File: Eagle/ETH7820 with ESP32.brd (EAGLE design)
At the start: 75 x 29.5 mm, 40 parts

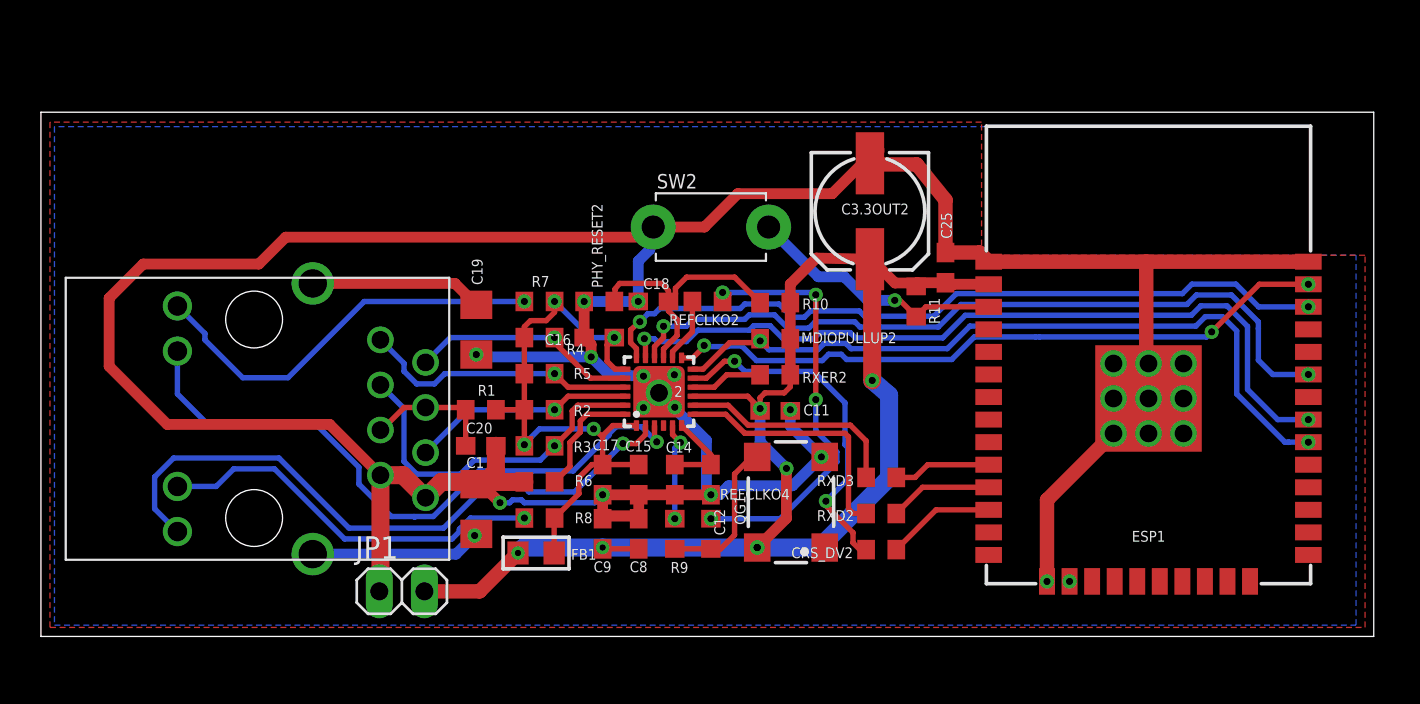
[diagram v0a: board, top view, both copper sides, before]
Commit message: board renew
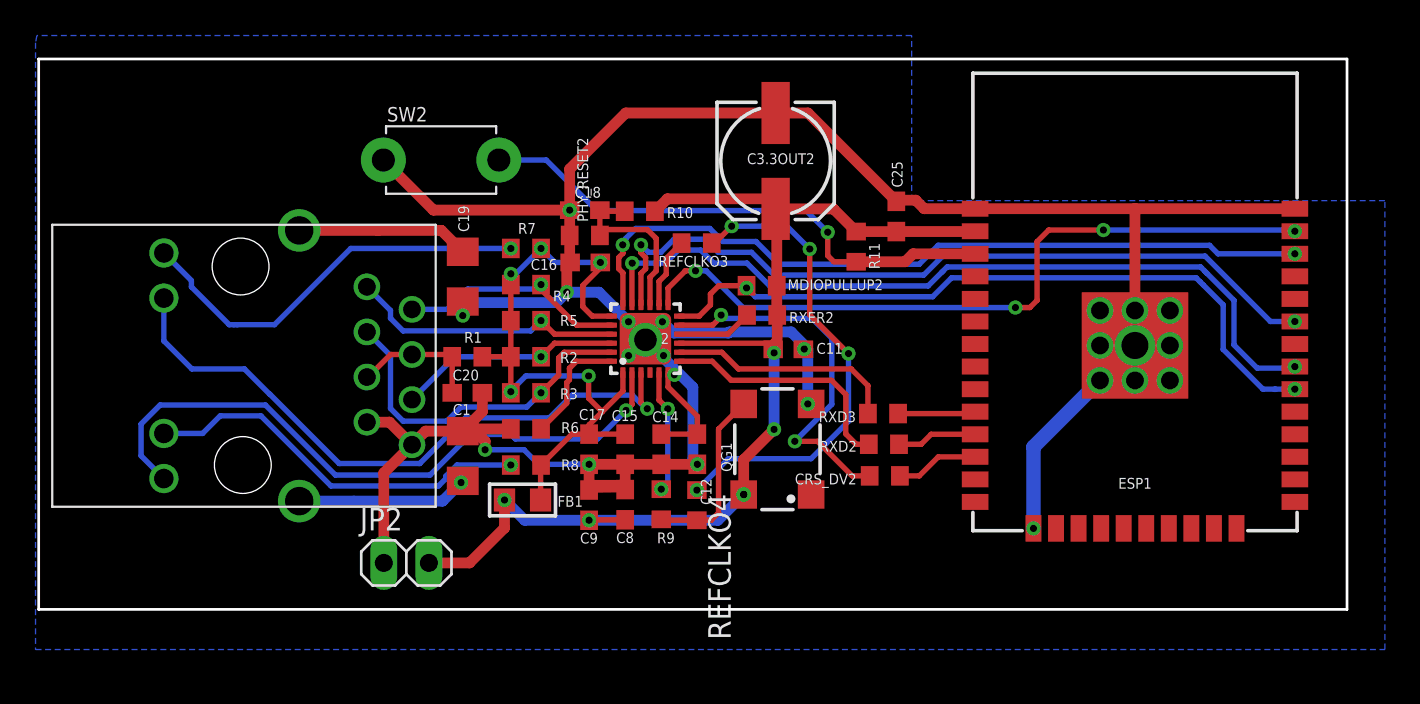
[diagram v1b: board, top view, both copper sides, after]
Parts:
- removed JP1: (no value), pinhead:1X02
- removed REFCLKO2: 33R/1%/R0603, rcl:R0603
- added JP2: (no value), pinhead:1X02
- added REFCLKO3: 33R/1%/R0603, rcl:R0603
- PHY_RESET2: value no value -> do not populate
- moved SW2 15.7 mm to (22.5, 26.8)
- moved R10 9.19 mm to (33.7, 23.9)
- moved C18 6.43 mm to (30.6, 24.0)
- moved C3.3OUT2 6.02 mm to (41.4, 26.8)
- moved R11 4.58 mm to (45.9, 21.9)
- moved C16 4.30 mm to (30.6, 21.1)
- moved CRS_DV2 4.16 mm to (47.5, 9.04)
- moved C25 4.00 mm to (48.2, 23.6)
- moved RXD2 3.90 mm to (47.5, 10.8)
- moved PHY_RESET2 3.81 mm to (30.6, 22.6)
- moved RXD3 3.60 mm to (47.4, 12.5)
- moved C11 3.54 mm to (42.1, 16.2)
- moved RXER2 3.45 mm to (40.6, 18.1)
- moved C19 3.08 mm to (23.7, 20.3)
- moved FB1 3.08 mm to (27.1, 7.68)
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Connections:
- removed net N$12 (its old number): 2.14, REFCLKO2.2
- removed net N$22 (its old number): REFCLKO2.1, REFCLKO4.1
- new net N$11: 2.14, REFCLKO3.2
- new net N$21: REFCLKO3.1, REFCLKO4.1
- net +3V3: now also JP2.2; no longer JP1.2
- net GND: now also JP2.1; no longer JP1.1
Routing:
- net GND: track 230.0 -> 199.4 mm
- net N$21: track 0.00 -> 27.3 mm, vias 0 -> 4
- net N$22 (its old number): track 24.3 -> 0.00 mm, vias 4 -> 0
- net EN: track 14.7 -> 30.1 mm
- net +3V3: track 81.4 -> 66.2 mm, vias 7 -> 6
- net N$15: track 14.9 -> 10.1 mm
- net N$11: track 0.00 -> 4.01 mm
- net N$12 (its old number): track 3.64 -> 0.00 mm
- net GPIO23: track 38.0 -> 41.4 mm, vias 3 -> 4
- net N$7: track 35.1 -> 38.2 mm, vias 4 -> 5
- net GPIO27: track 6.13 -> 4.68 mm
- net N$9: track 5.56 -> 6.92 mm
- net N$23: track 8.79 -> 10.1 mm
- net GPIO26: track 5.81 -> 4.52 mm
- net N$8: track 4.91 -> 6.18 mm
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- removed copper zone on layer 1, net GND
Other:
- board size 75 x 29.5 mm -> 73.7 x 31 mm
- board text added: "+3V"
- board text added: "ESP32"
- board text added: "GND"
- board text added: "KEEPOUT"
- board text added: "RST"
